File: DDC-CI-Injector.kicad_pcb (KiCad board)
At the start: 4 copper layers, 49.1 x 39.3 mm, 25 parts, among them J1 HDMI_A, J2 HDMI_A, J3 Connector, U1 PCA9641, U2 XC6206PxxxMR, U3 PCA9509, U4 PCA9509, U5 ESD224DQA, U6 ESD224DQA, U7 ESD224DQA

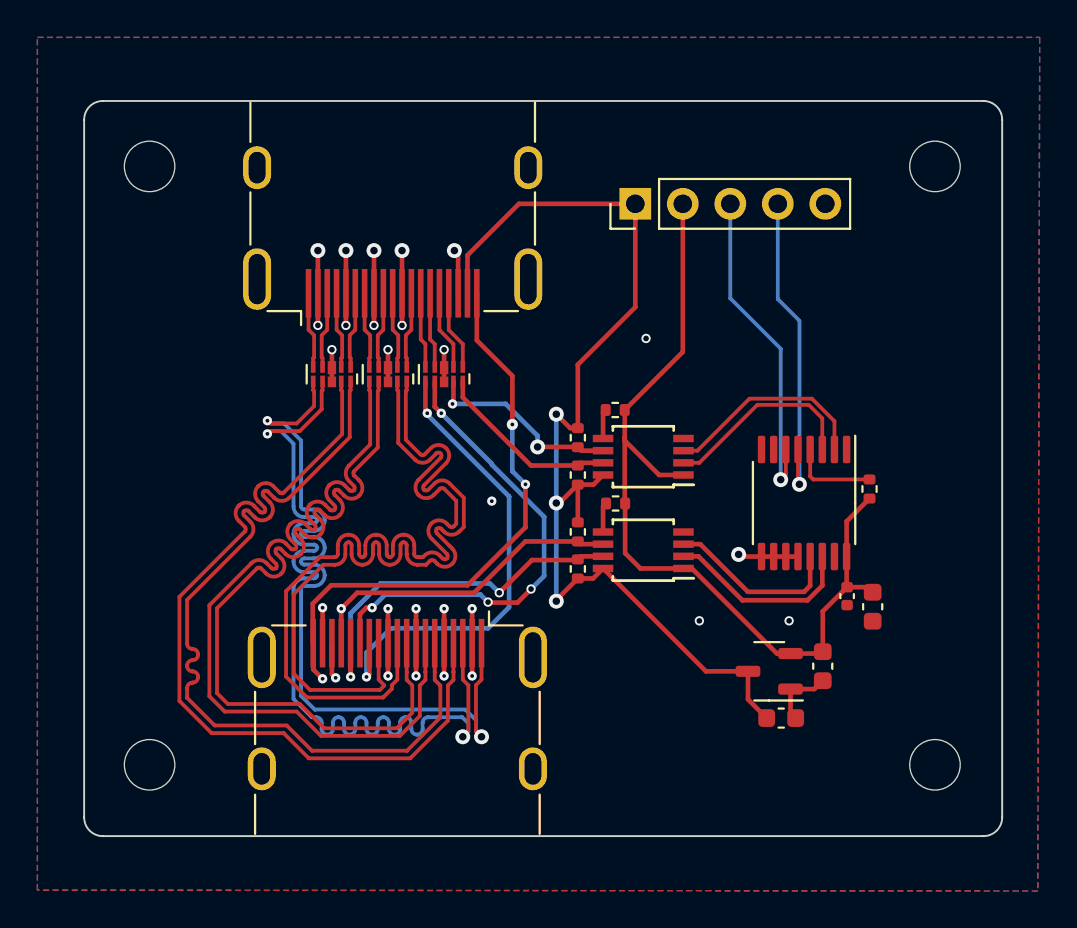
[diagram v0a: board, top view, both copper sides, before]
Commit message: Better routing
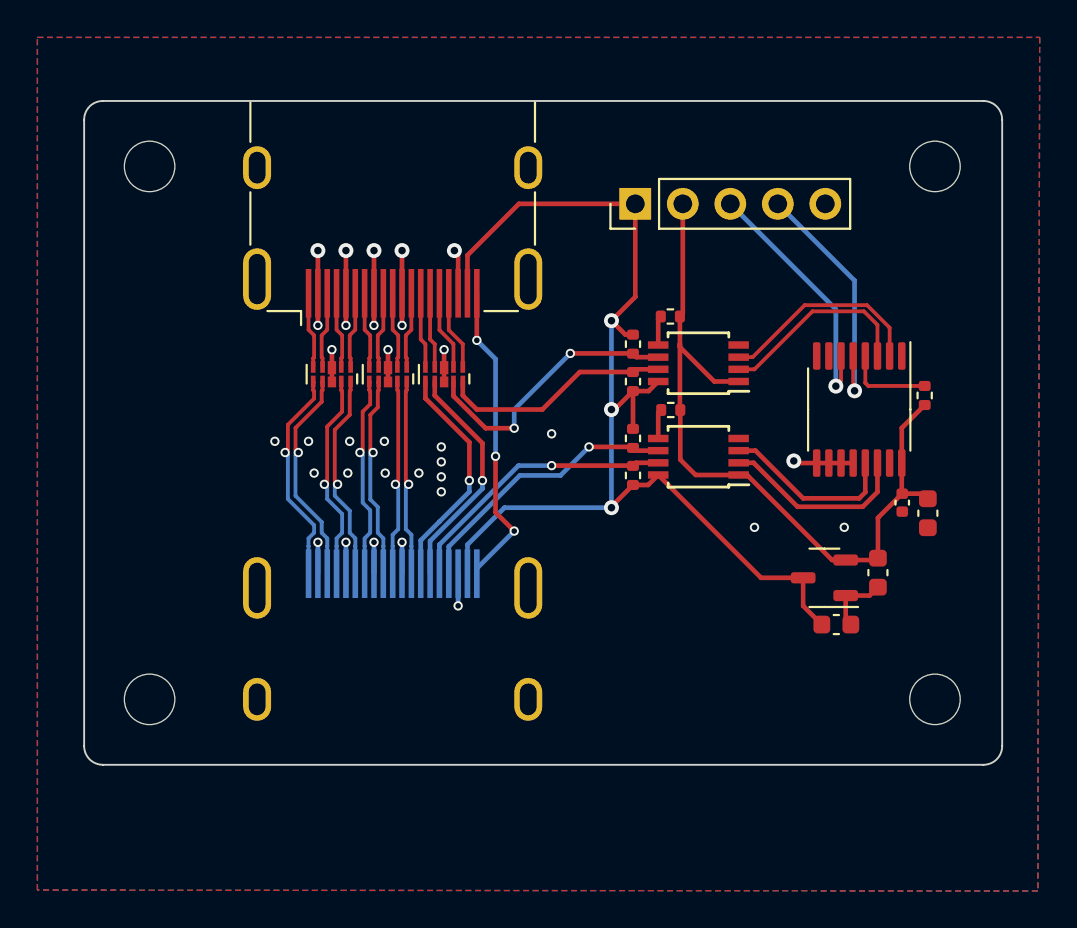
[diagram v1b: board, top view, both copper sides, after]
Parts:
- J2: moved to B.Cu
- moved R2 5.81 mm to (101.9, 60.5)
- moved C2 5.81 mm to (113.0, 69.2)
- moved C4 5.81 mm to (114.2, 65.5)
- moved R7 5.81 mm to (115.5, 59.8)
- moved U1 5.81 mm to (112.0, 60.5)
- moved U2 5.81 mm to (110.1, 69.5)
- moved U4 5.81 mm to (103.3, 63.0)
- moved C1 5.81 mm to (110.7, 72.0)
- moved C3 5.81 mm to (115.6, 66.0)
- moved R1 5.81 mm to (101.8, 55.5)
- moved R3 5.81 mm to (99.8, 64.0)
- moved R4 5.81 mm to (99.8, 62.0)
- moved R5 5.81 mm to (99.8, 57.0)
- moved U3 5.81 mm to (103.3, 58.0)
- moved R6 5.81 mm to (99.8, 59.0)
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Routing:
- net /D2_B-: track 47.9 -> 11.8 mm, vias 2 -> 1
- net /CK_B+: track 44.6 -> 10.5 mm, vias 0 -> 1
- net /D0_B+: track 44.7 -> 10.9 mm, vias 0 -> 1
- net /D1_B+: track 44.9 -> 11.2 mm, vias 0 -> 1
- net /D1_B-: track 44.8 -> 11.2 mm, vias 0 -> 1
- net /CK_B-: track 43.3 -> 10.5 mm, vias 0 -> 1
- net /D0_B-: track 43.4 -> 10.9 mm, vias 0 -> 1
- net /D2_B+: track 41.8 -> 11.8 mm, vias 2 -> 1
- net Net-(J1-HPD): track 30.9 -> 16.7 mm
- net Net-(J2-CEC): track 25.7 -> 12.3 mm, vias 2 -> 1
- net Net-(J2-UTILITY): track 25.4 -> 12.5 mm, vias 4 -> 1
- net GND: track 46.2 -> 38.3 mm, vias 26 -> 33
- net +3V3: track 47.0 -> 40.8 mm
- net Net-(J2-SCL): track 20.3 -> 15.1 mm, vias 2 -> 1
- net Net-(U3-B1): track 10.6 -> 14.8 mm
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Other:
- board size 49.1 x 39.3 mm -> 49.1 x 35.5 mm
